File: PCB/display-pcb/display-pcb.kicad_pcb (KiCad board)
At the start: 2 copper layers, 128 x 57 mm, 9 parts, among them J1 B6B-XH-A, J2 B8B-XH-A, SW0 PTS645SL50-2 LFS, SW1 PTS645SL50-2 LFS, SW2 PTS645SL50-2 LFS, SW3 PTS645SL50-2 LFS, U1 NHD-C12864A1Z

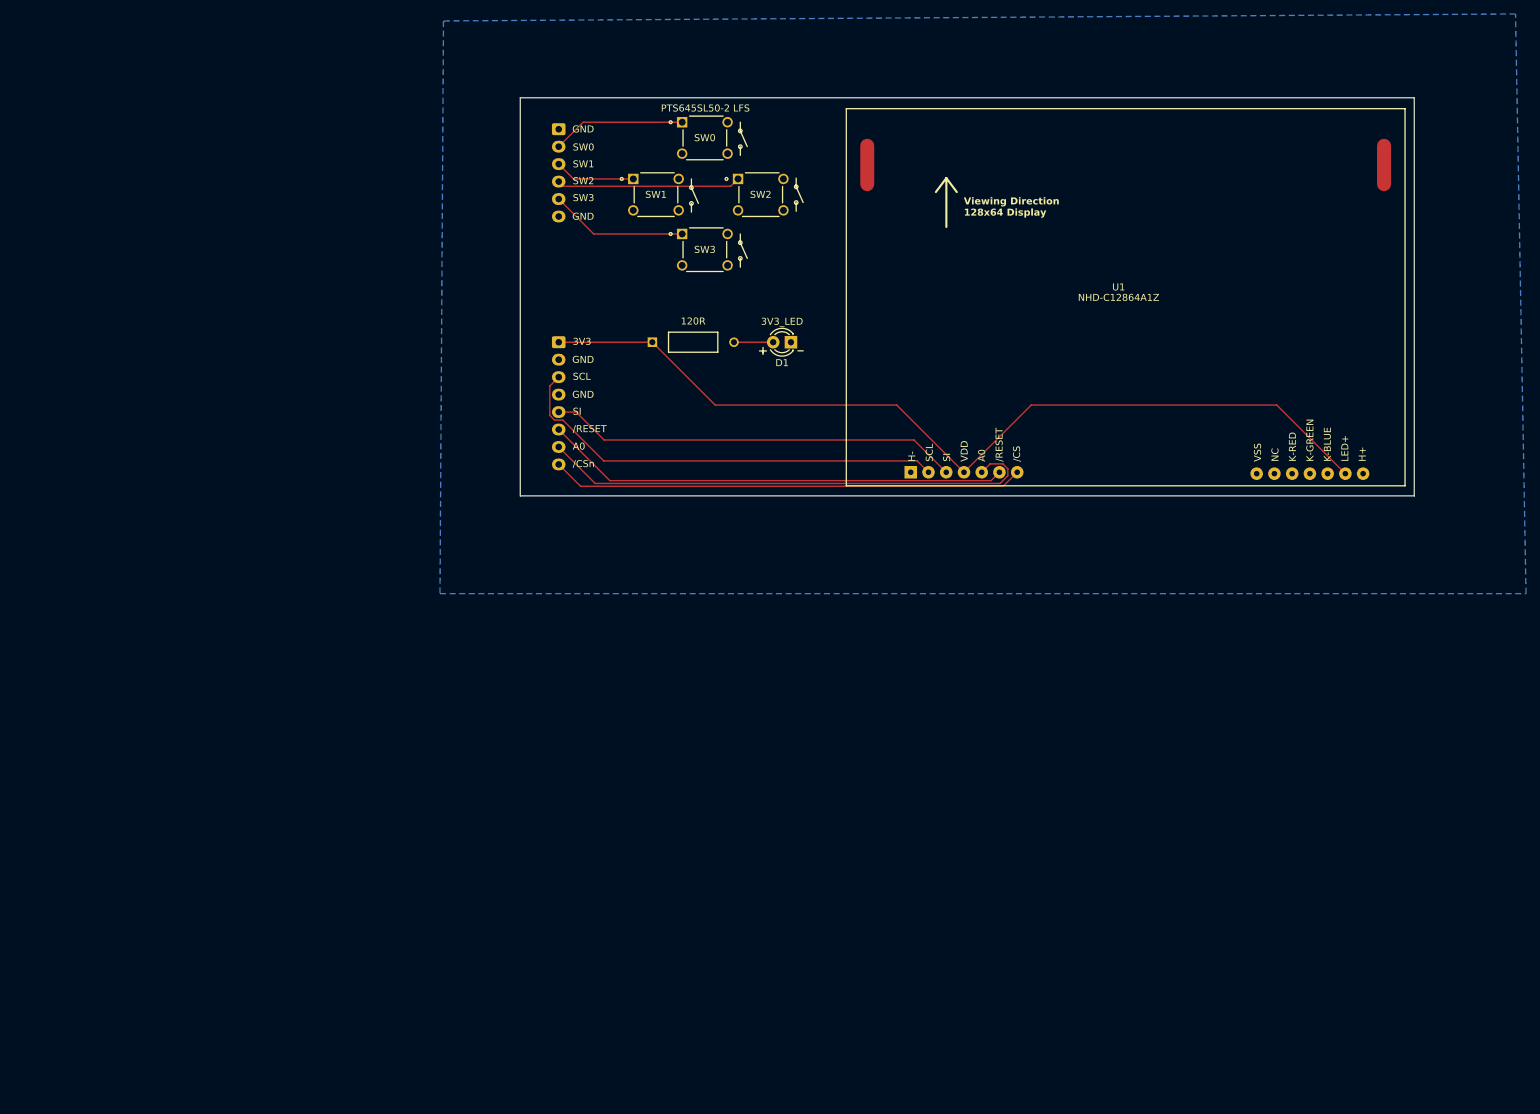
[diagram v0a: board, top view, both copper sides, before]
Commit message: PCB updates
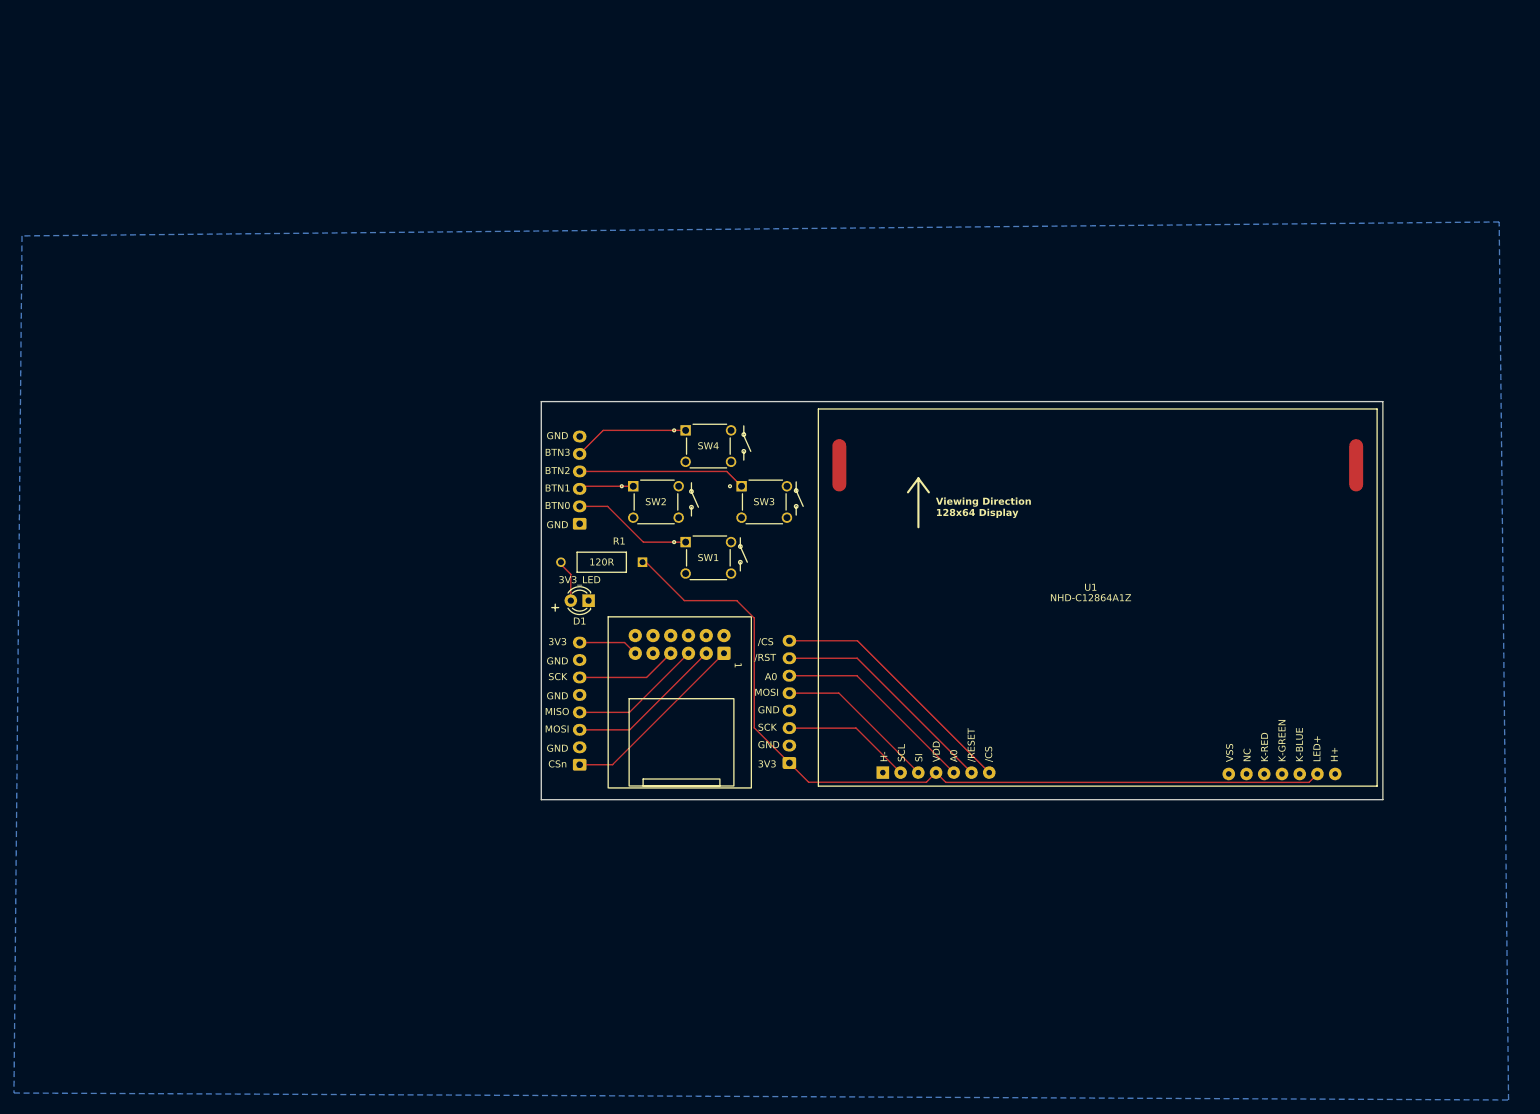
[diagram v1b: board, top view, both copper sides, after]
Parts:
- removed SW0: PTS645SL50-2 LFS, footprints:PTS654S_CNK
- added J3: B8B-XH-A, Connector_JST:JST_XH_B8B-XH-A_1x08_P2.50mm_Vertical, B.Cu at (125.5, 121.5)
- added SW4: PTS645SL50-2 LFS, footprints:PTS654S_CNK, F.Cu at (140.7, 73.6)
- added U2: ~, microsd:pmod-microsd, F.Cu at (140.1, 114.5)
- moved J2 68.7 mm to (155.5, 121.2), turned to 90 degrees
- moved J1 56.6 mm to (125.5, 87.0), turned to 90 degrees
- moved SW1 52.5 mm to (140.7, 89.6)
- moved D1 47.0 mm to (126.8, 98.0)
- moved SW2 46.5 mm to (133.2, 81.6)
- moved U1 43.2 mm to (198.7, 96.6)
- moved SW3 37.1 mm to (148.7, 81.6)
- moved R1 31.5 mm to (134.5, 92.5), turned to 180 degrees
- renumbered 120R to R1
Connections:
- J2 pad 6: /RESET -> A0
- J2 pad 7: A0 -> /RESET
- SW1 pad 1: BTN1 -> BTN0
- SW2 pad 1: BTN2 -> BTN1
- SW3 pad 1: BTN3 -> BTN2
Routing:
- net SCL: track 63.6 -> 18.6 mm
- net A0: track 72.5 -> 29.3 mm
- net SI: track 59.1 -> 23.2 mm
- net /RESET: track 66.6 -> 32.9 mm
- net /CS: track 67.8 -> 36.4 mm
- net SD_CSn: track 0.00 -> 27.3 mm
- net SD_MOSI: track 0.00 -> 22.7 mm
- net SD_MISO: track 0.00 -> 19.1 mm
- net SD_SCK: track 0.00 -> 14.5 mm
- net SD_3V3: track 0.00 -> 8.60 mm
- net 3V3: track 129.1 -> 120.5 mm
- net BTN1: track 11.6 -> 7.83 mm
- net BTN3: track 19.7 -> 16.6 mm
- net BTN2: track 26.4 -> 24.1 mm
- net BTN0: track 19.1 -> 17.3 mm
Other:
- board size 128 x 57 mm -> 120.5 x 57 mm
- board text added: "/CS"
- board text added: "/RST"
- board text added: "BTN0"
- board text added: "BTN1"
- board text added: "BTN2"
- board text added: "BTN3"
- board text added: "CSn"
- board text added: "MISO"
- board text added: "MOSI"
- board text added: "SCK"
- board text removed: "/CSn"
- board text removed: "/RESET"
- board text removed: "SCL"
- board text removed: "SI"
- board text removed: "SW0"
- board text removed: "SW1"
- board text removed: "SW2"
- board text removed: "SW3"
